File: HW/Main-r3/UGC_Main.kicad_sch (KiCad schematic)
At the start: 137 parts, among them J1 SM02B-SURS-TF_LF__SN_, J13 503480-0640, J2 LT, J3 RT, J4 Conn_01x06_Pin, J5 UJ31-CH-G1-SMT-TR, J8 Conn_01x02, J9 Conn_01x02, Q1 MMBT3904, Q2 MMBT3904, Q3 BSS138DW, Q4 BSS138DW, Q5 Q_NMOS_GSD, SW1 1TS026A-1000-0550, SW1 SW_Push, SW10 SW_Push, SW11 SW_Push, SW12 SW_Push, SW13 SW_Push, SW14 TS09-63-25-R-260-SMT, SW17 TS09-63-25-R-260-SMT, SW18 TS09-63-25-R-260-SMT, SW19 TS09-63-25-R-260-SMT, SW2 SW_Push, SW20 TS09-63-25-R-260-SMT, SW3 SW_Push, SW4 SW_Push, SW6 GL18_SW, SW7 SW_Push, SW8 SW_Push, SW9 TS09-63-25-R-260-SMT, U1 ESP32-PICO-MINI-02, U10 ST_LSM6, U11 BQ25180, U12 CH340K, U13 PI3USB4000A, U2 GD25Q80EEIGR, U2 GH39F (Hall SOT23), U3 GH39F (Hall SOT23), U4 TPS630001RCR, U5 ST_LSM6, U6 MCP3002, U7 MCP3002, U8 RP2040, Y1 Crystal_GND3

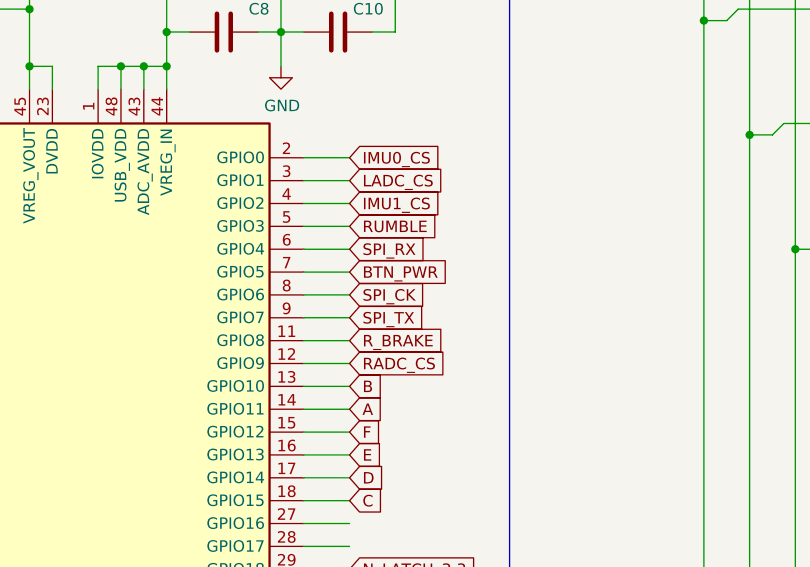
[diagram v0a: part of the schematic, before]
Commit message: Update revision
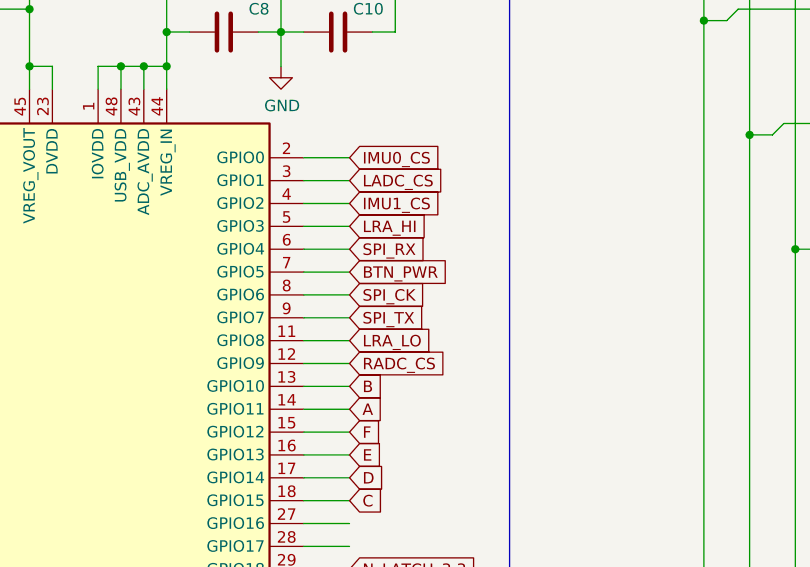
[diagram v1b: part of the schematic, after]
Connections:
- net RUMBLE is gone; now on net LRA_HI: U8.5 (GPIO3)
- net R_BRAKE is gone; now on net LRA_HI: U8.11 (GPIO8)
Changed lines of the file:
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@@
 		)
 	)
-	(global_label "RUMBLE"
+	(global_label "LRA_HI"
 		(shape input)
 		(at 388.62 166.37 0)
@@
 		)
 		(property "Intersheetrefs" "${INTERSHEET_REFS}"
-			(at 398.4432 166.4494 0)
+			(at 397.8948 166.37 0)
 			(effects
 				(font
@@
 		)
 	)
-	(global_label "R_BRAKE"
+	(global_label "LRA_LO"
 		(shape input)
 		(at 388.62 179.07 0)
@@
 		)
 		(property "Intersheetrefs" "${INTERSHEET_REFS}"
-			(at 399.2294 179.1494 0)
-			(effects
-				(font
+			(at 398.3181 179.07 0)
+			(effects
+				(font
